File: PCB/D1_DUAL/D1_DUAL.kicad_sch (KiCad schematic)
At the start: 34 parts, among them J1 Conn_01x03, J11 Conn_01x02, J5 Conn_01x04_Pin, J7 Conn_01x04, J8 Conn_01x03, J9 Conn_01x03

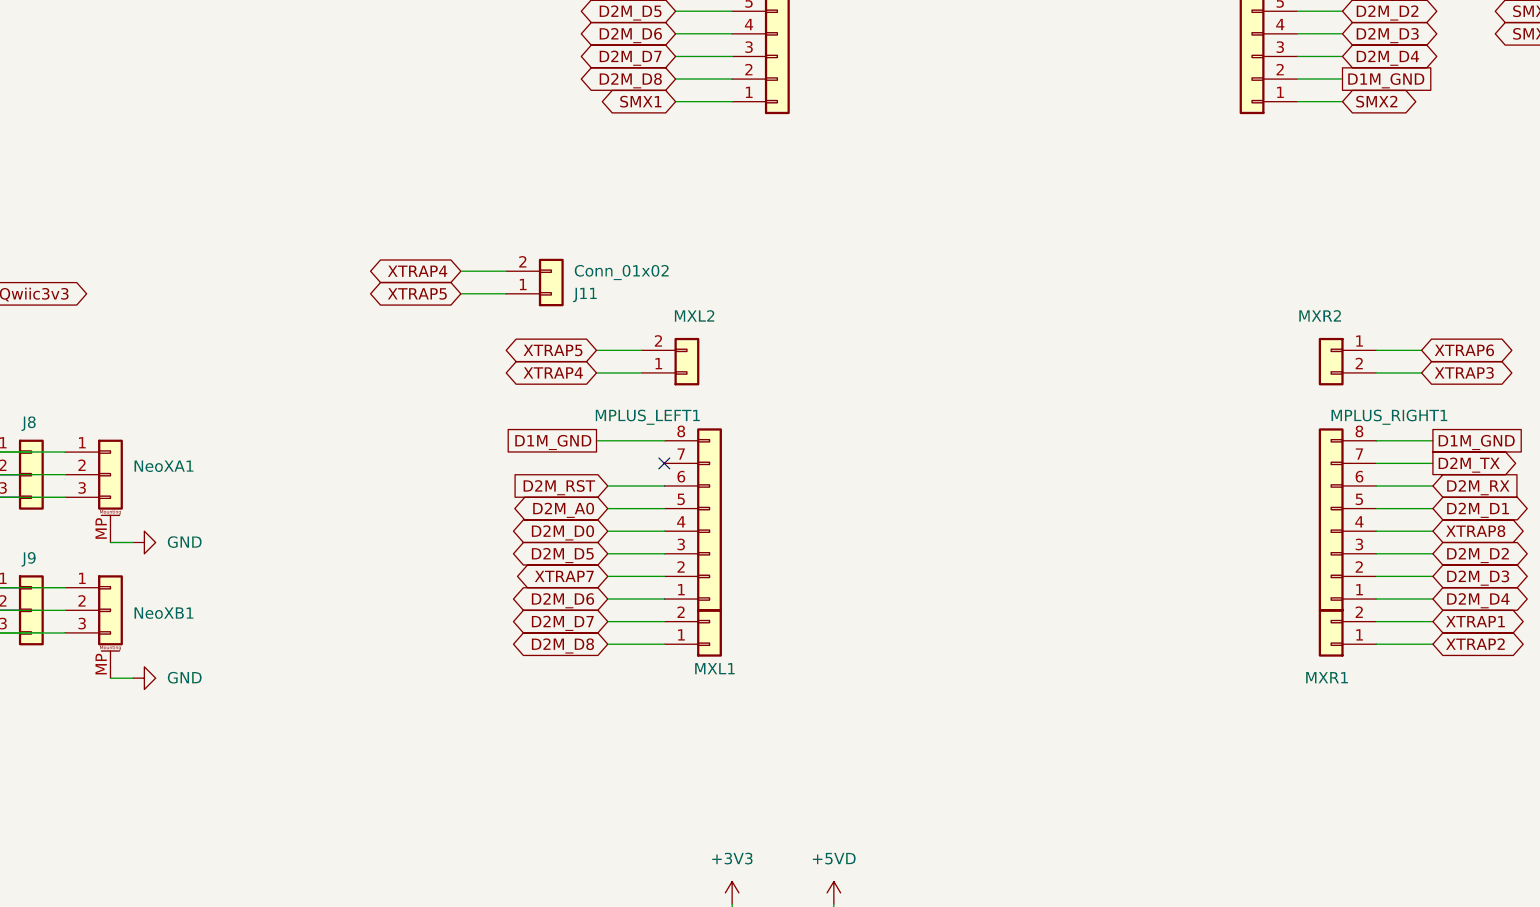
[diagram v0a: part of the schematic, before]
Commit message: Working on Treasure Chest Demo
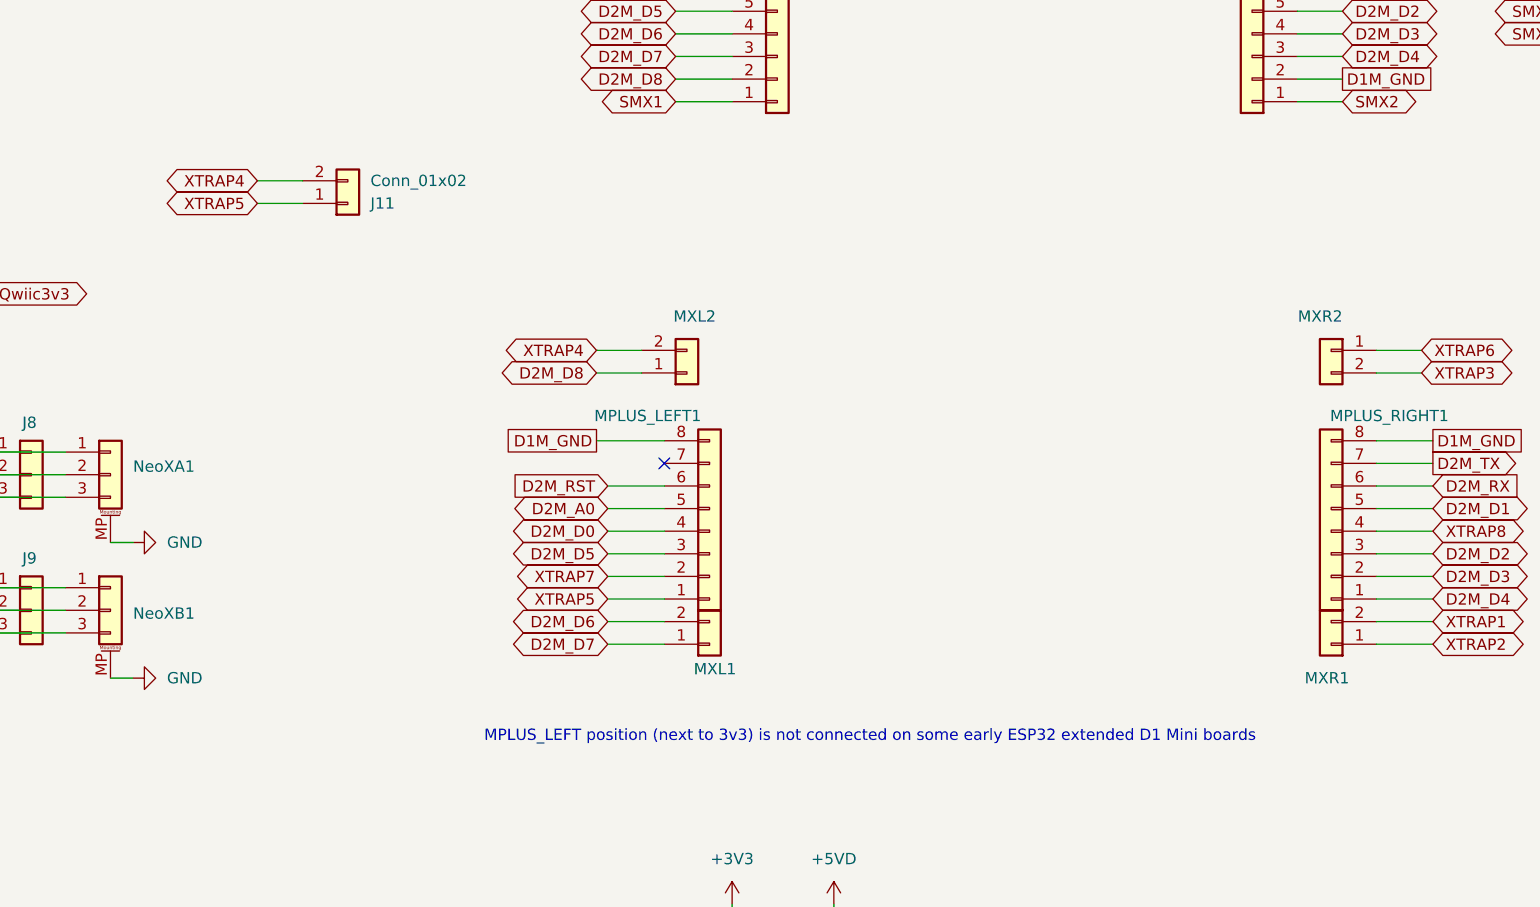
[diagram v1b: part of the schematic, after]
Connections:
- net D2M_D6: now also MXL1.2 (Pin_2); no longer MPLUS_LEFT1.1 (Pin_1)
- net D2M_D7: now also MXL1.1 (Pin_1); no longer MXL1.2 (Pin_2)
- net D2M_D8: now also MXL2.1 (Pin_1); no longer MXL1.1 (Pin_1)
- net XTRAP4: now also MXL2.2 (Pin_2); no longer MXL2.1 (Pin_1)
- net XTRAP5: now also MPLUS_LEFT1.1 (Pin_1); no longer MXL2.2 (Pin_2)
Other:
- note added: "MPLUS_LEFT position (next to 3v3) is not connected on some early ESP32 extended D1 Mini boards"
- company: (none) -> Lumensalis
- title: (none) -> ESP32 D1 Double Base
- moved on the sheet: J11
